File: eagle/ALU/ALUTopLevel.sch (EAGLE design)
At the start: 0 parts

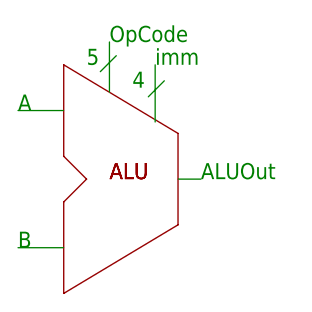
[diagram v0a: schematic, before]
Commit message: Schematics small improvements
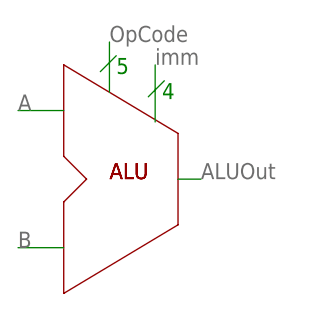
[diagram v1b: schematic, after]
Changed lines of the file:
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@@
 <setting verticaltext="up"/>
 </settings>
-<grid distance="0.1" unitdist="inch" unit="inch" style="lines" multiple="1" display="yes" altdistance="0.01" altunitdist="inch" altunit="inch"/>
+<grid distance="0.1" unitdist="inch" unit="inch" style="lines" multiple="1" display="no" altdistance="0.01" altunitdist="inch" altunit="inch"/>
 <layers>
 <layer number="91" name="Nets" color="2" fill="1" visible="yes" active="yes"/>
@@
 <text x="12.7" y="66.04" size="1.778" layer="94">ALU</text>
 <text x="12.7" y="66.04" size="1.778" layer="94">ALU</text>
-<text x="22.86" y="66.04" size="1.778" layer="91">ALUOut</text>
-<text x="2.54" y="58.42" size="1.778" layer="91">B</text>
-<text x="2.54" y="73.66" size="1.778" layer="91">A</text>
-<text x="12.7" y="81.28" size="1.778" layer="91">OpCode</text>
-<text x="10.16" y="78.74" size="1.778" layer="91">5</text>
-<text x="15.24" y="76.2" size="1.778" layer="91">4</text>
-<text x="17.78" y="78.74" size="1.778" layer="91">imm</text>
+<text x="22.86" y="66.04" size="1.778" layer="95">ALUOut</text>
+<text x="2.54" y="58.42" size="1.778" layer="95">B</text>
+<text x="2.54" y="73.66" size="1.778" layer="95">A</text>
+<text x="12.7" y="81.28" size="1.778" layer="95">OpCode</text>
+<text x="13.462" y="77.724" size="1.778" layer="91">5</text>
+<text x="18.542" y="74.93" size="1.778" layer="91">4</text>
+<text x="17.78" y="78.74" size="1.778" layer="95">imm</text>
 </plain>
 <instances>
